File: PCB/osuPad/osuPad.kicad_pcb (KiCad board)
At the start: 2 copper layers, 66 x 81 mm, 11 parts, among them SW1 SW_Push, SW2 SW_Push, SW3 SW_Push, SW4 SW_Push, SW5 SW_Push, SW6 SW_Push, SW7 SW_Push, SW8 SW_Push, SW9 SW_Push, U1 XIAO-RP2040-DIP

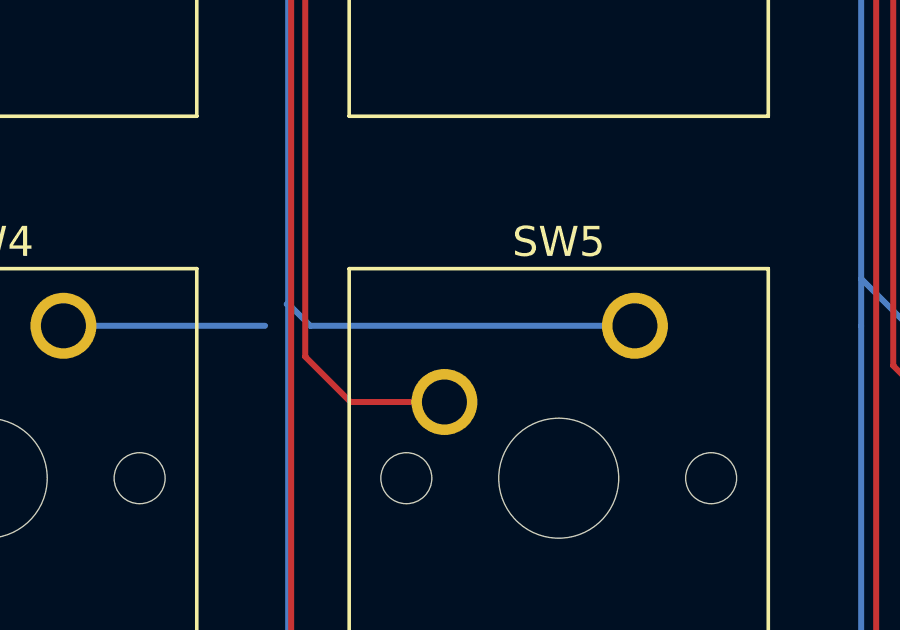
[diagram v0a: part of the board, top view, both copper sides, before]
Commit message: update image
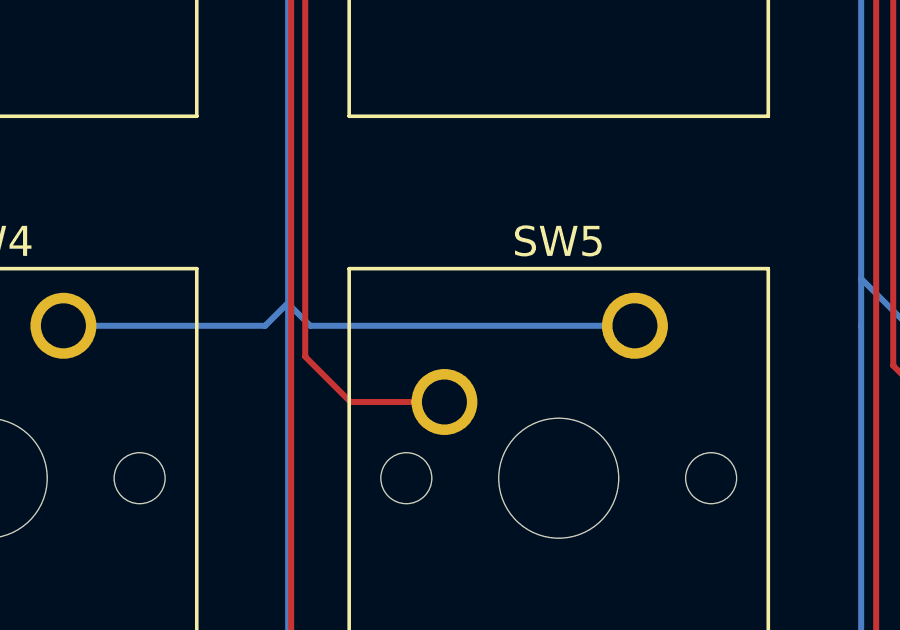
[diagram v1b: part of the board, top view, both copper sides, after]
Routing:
- net GND: track 246.1 -> 247.0 mm
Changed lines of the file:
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@@
-	)
-	(segment
-		(start 137.25125 67.84875)
-		(end 136.13125 67.84875)
-		(width 0.2)
-		(layer "B.Cu")
-		(net 3)
 	)
 	(segment
@@
 	)
 	(segment
-		(start 124.68125 104.95)
-		(end 124.75 104.95)
+		(start 137.25125 67.84875)
+		(end 136.13125 67.84875)
 		(width 0.2)
 		(layer "B.Cu")
@@
 	)
 	(segment
+		(start 123.96125 105.67)
+		(end 124.68125 104.95)
+		(width 0.2)
+		(layer "B.Cu")
+		(net 3)
+	)
+	(segment
 		(start 155.29125 124.76875)
 		(end 155.34 124.72)
@@
 	)
 	(segment
-		(start 136.29 86.62)
-		(end 125.35125 86.62)
+		(start 136.29 105.67)
+		(end 125.47 105.67)
 		(width 0.2)
 		(layer "B.Cu")
@@
 	)
 	(segment
-		(start 125.47 105.67)
-		(end 136.29 105.67)
+		(start 136.29 86.62)
+		(end 125.35125 86.62)
 		(width 0.2)
 		(layer "B.Cu")

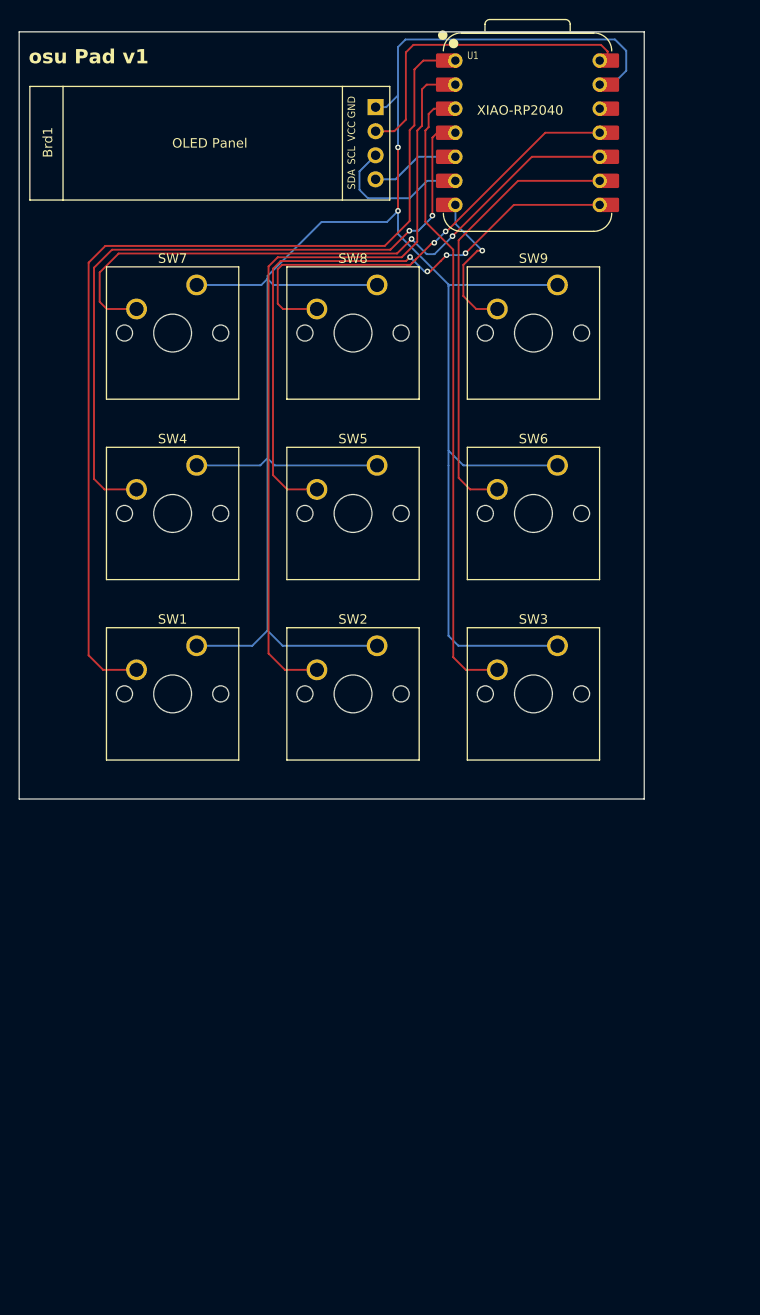
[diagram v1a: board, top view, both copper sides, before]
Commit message: add journal
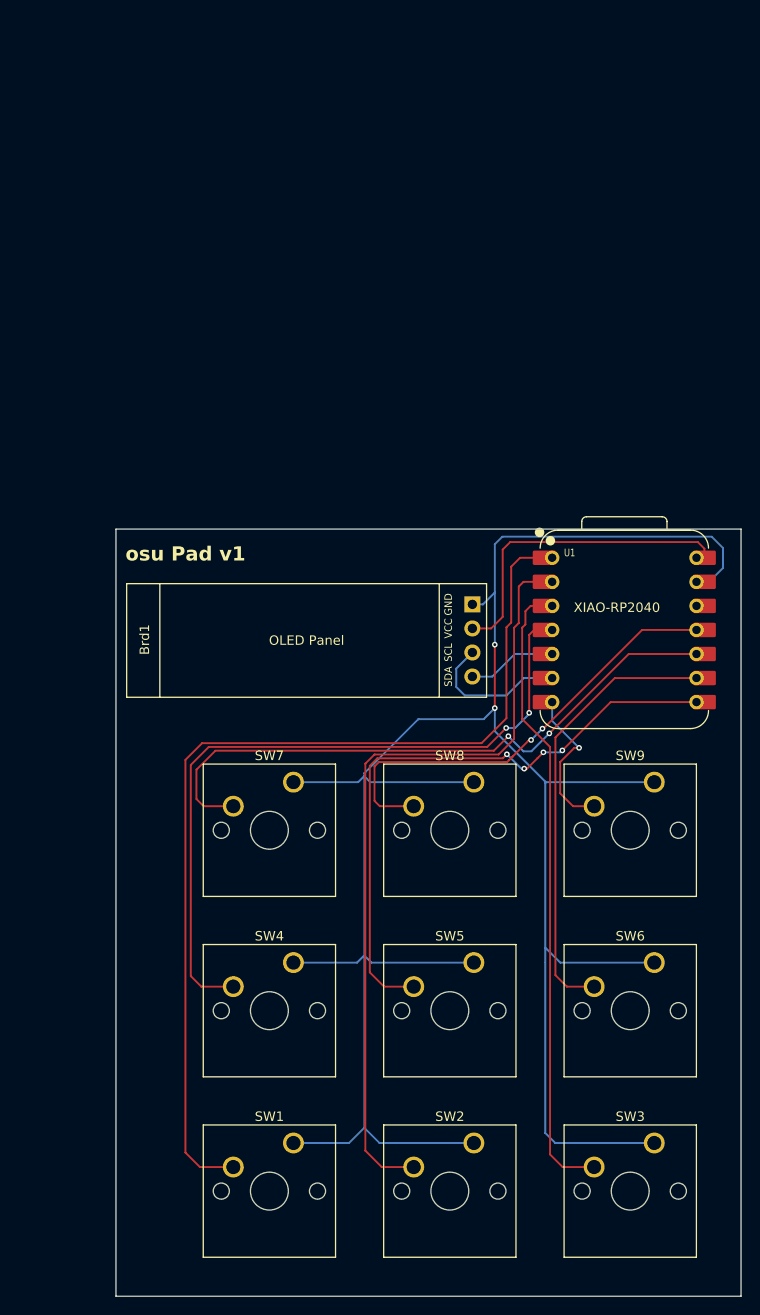
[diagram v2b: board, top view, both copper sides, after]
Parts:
- moved Brd1 53.5 mm to (109.9, 118.2)
- moved SW1 53.5 mm to (127.5, 177.2)
- moved SW2 53.5 mm to (146.5, 177.2)
- moved SW3 53.5 mm to (165.6, 177.2)
- moved SW7 53.5 mm to (127.5, 139.1)
- moved SW8 53.5 mm to (146.5, 139.1)
- moved SW9 53.5 mm to (165.6, 139.1)
- moved U1 53.5 mm to (162.4, 123.0)
- moved SW4 53.5 mm to (127.5, 158.2)
- moved SW5 53.5 mm to (146.5, 158.2)
- moved SW6 53.5 mm to (165.6, 158.2)
